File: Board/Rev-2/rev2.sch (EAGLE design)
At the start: 60 parts, among them IC1 74HC595N, T1 2N3904, T2 2N3904, T3 2N3904, T4 2N3904, T5 2N3904, T6 2N3904, T7 2N3904, T8 2N3904

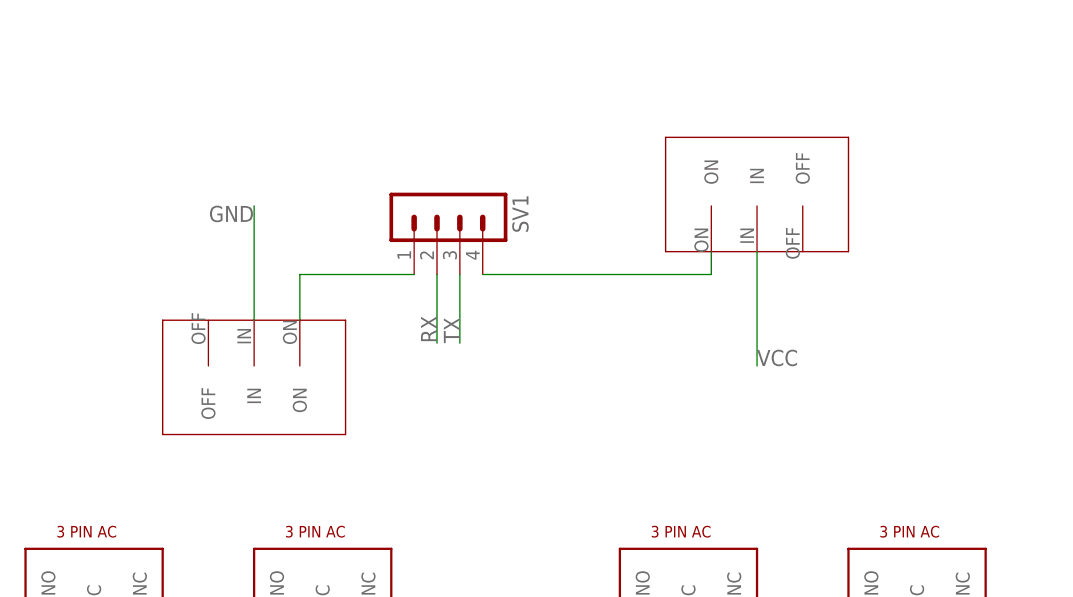
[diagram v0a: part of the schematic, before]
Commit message: board updated
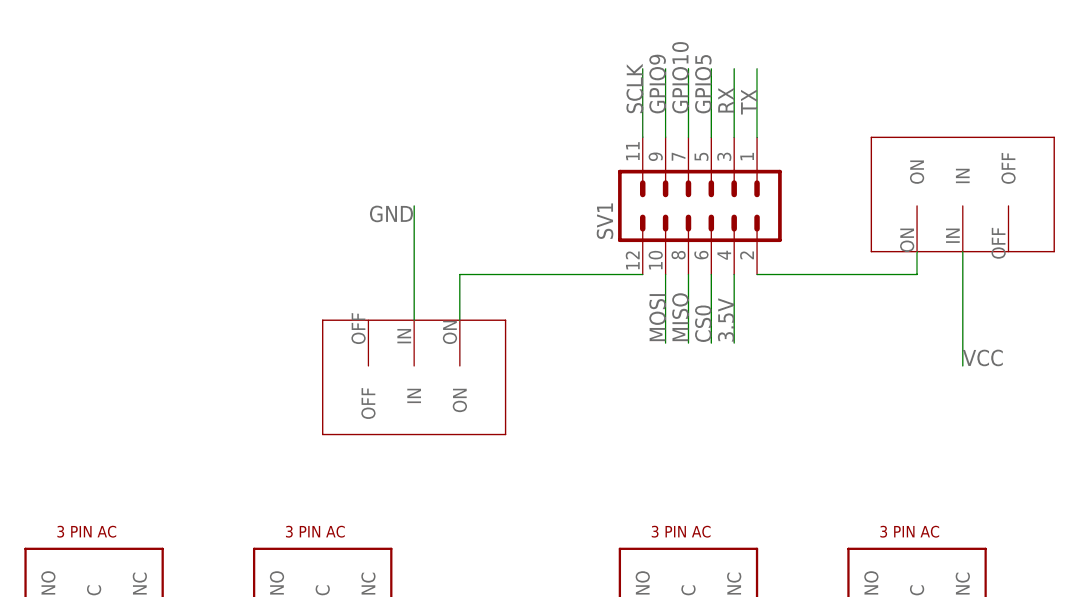
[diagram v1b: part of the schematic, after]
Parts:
- SV1: device con-lstb:MA04-1 -> con-lstb:MA06-2
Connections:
- net 3.5V: now also SV1.4
- net CS0: now also SV1.6
- net GPIO10: now also SV1.7
- net GPIO5: now also SV1.5
- net GPIO9: now also SV1.9
- net MISO: now also SV1.8
- net MOSI: now also SV1.10
- net N$55: now also SV1.12; no longer SV1.1
- net N$56: now also SV1.2; no longer SV1.4
- net RX: now also SV1.3; no longer SV1.2
- net SCLK: now also SV1.11
- net TX: now also SV1.1; no longer SV1.3
